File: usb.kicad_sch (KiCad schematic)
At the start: 3 parts, among them J1 USB_C_Receptacle_USB2.0

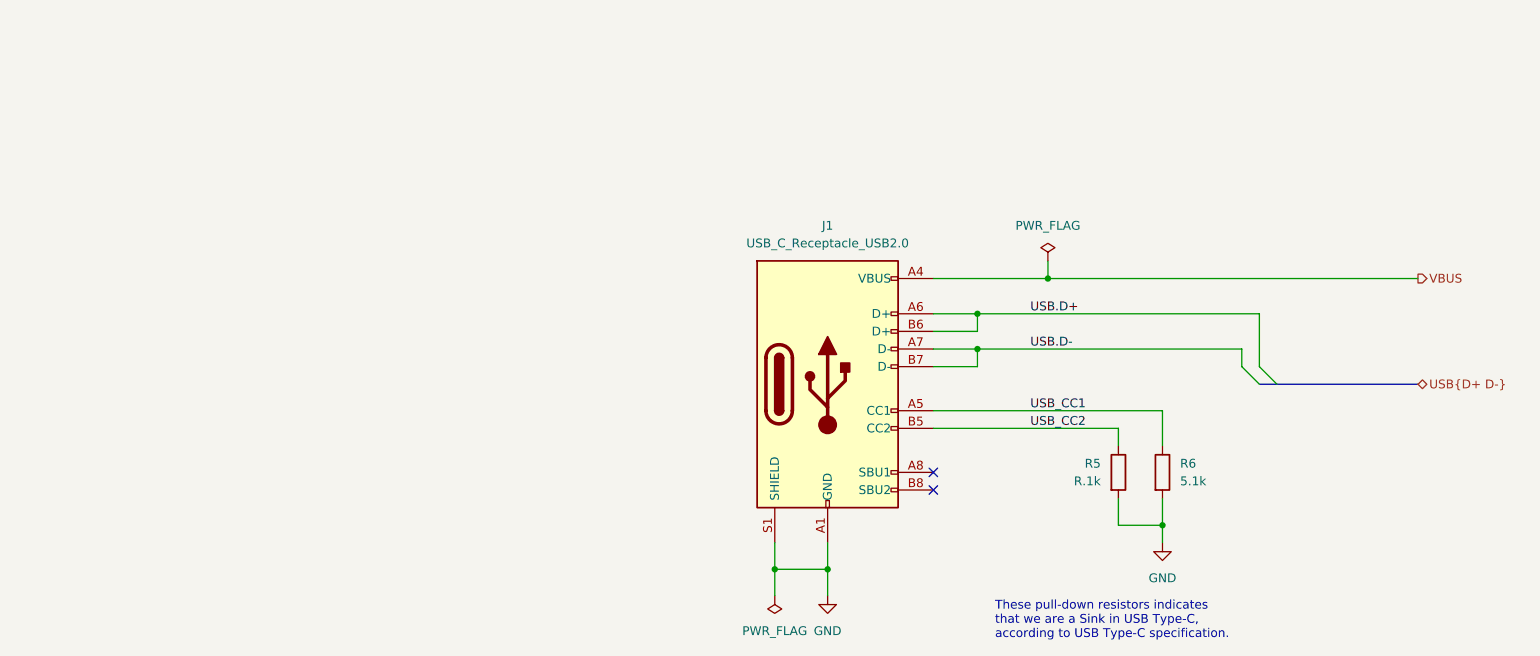
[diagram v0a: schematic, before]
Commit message: Big update, bad commit messsage :)
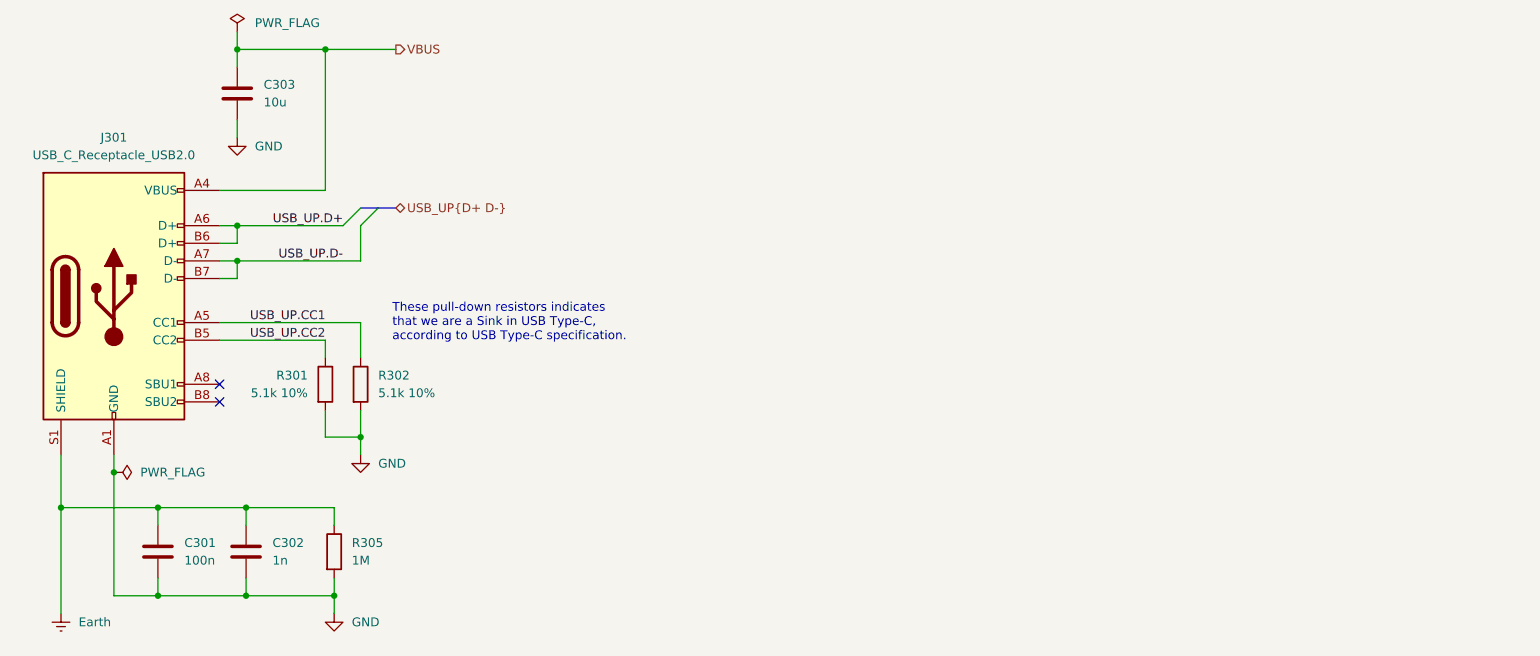
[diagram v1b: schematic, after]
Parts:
- added C301: 100n, cubesat_rp2040:C_0402_1005Metric, symbol Device:C
- added C302: 1n, cubesat_rp2040:C_0402_1005Metric, symbol Device:C
- added C303: 10u, cubesat_rp2040:C_0402_1005Metric, symbol Device:C
- added R305: 1M, cubesat_rp2040:R_0402_1005Metric, symbol Device:R
- R301: renamed from R5; value R.1k -> 5.1k 10%; footprint Resistor_SMD:R_0402_1005Metric -> cubesat_rp2040:R_0402_1005Metric
- R302: renamed from R6; value 5.1k -> 5.1k 10%; footprint Resistor_SMD:R_0402_1005Metric -> cubesat_rp2040:R_0402_1005Metric
- renumbered J1 to J301
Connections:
- net GND: now also C301.2, C302.2, C303.2, R305.2; no longer J301.S1 (SHIELD)
- net VBUS: now also C303.1
- net USB.D+ renamed USB_UP.D+
- net USB.D- renamed USB_UP.D-
- net USB_CC1 renamed USB_UP.CC1
- net USB_CC2 renamed USB_UP.CC2
- new net Earth: C301.1, C302.1, J301.S1 (SHIELD), R305.1
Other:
- company: (none) -> Magnus Oksbøl Therkelsen
- title: (none) -> CubeSat RP2040 Board
- moved on the sheet: J301, R301, R302
